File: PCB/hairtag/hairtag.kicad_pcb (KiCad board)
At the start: 2 copper layers, 24 x 24 mm, 19 parts, among them J1 Flash, J2 BAT, U1 ESP32-C3FH4, X1 XL2EL89CPI-111YLC-40M

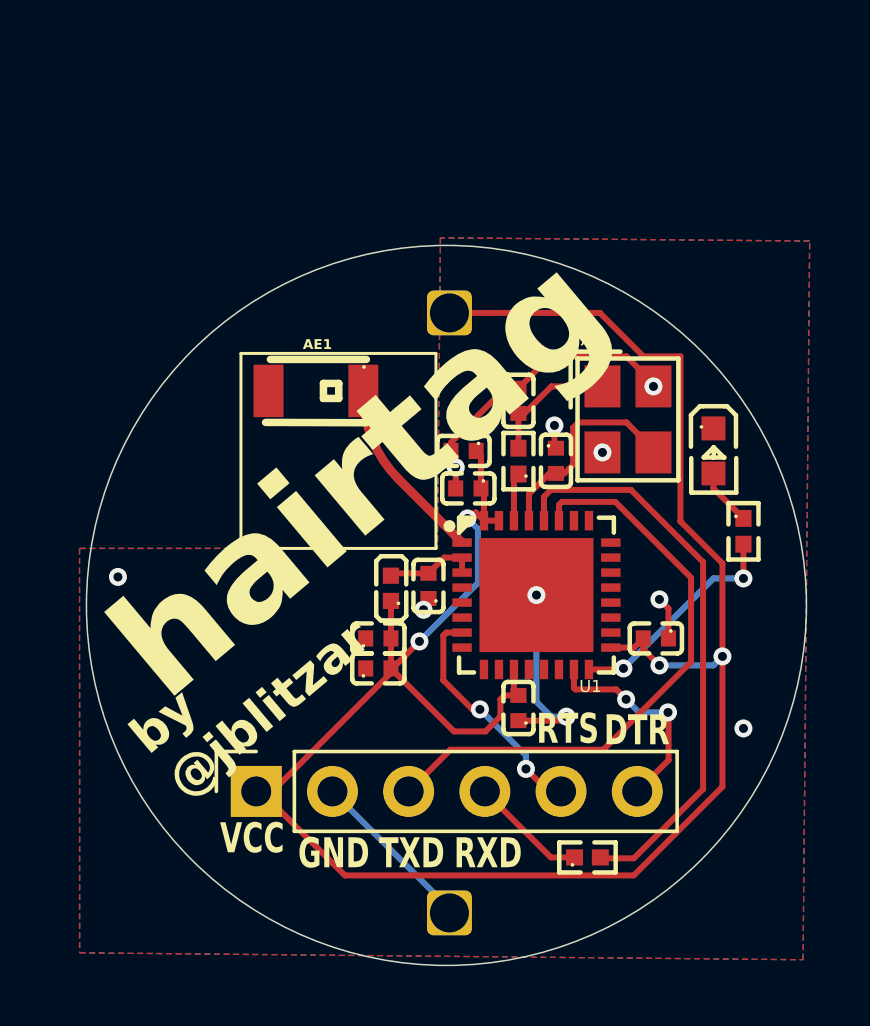
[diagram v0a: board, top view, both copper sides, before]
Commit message: tweaks
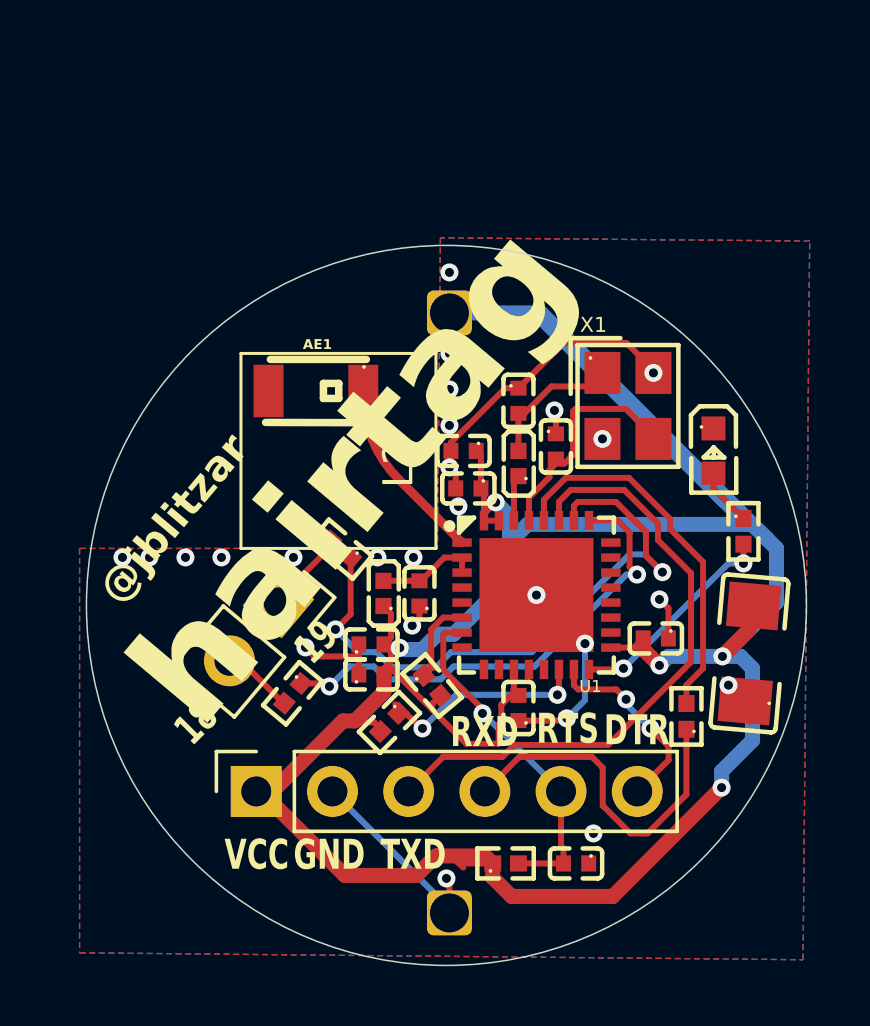
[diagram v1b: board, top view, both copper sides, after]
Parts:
- added C11: 100uF, lcsc:C1206, F.Cu at (65.2, 57.0)
- added C8: 1uF, lcsc:C0402, F.Cu at (59.4, 64.0)
- added L2: 15nH, lcsc:L0402, F.Cu at (57.5, 50.7)
- added R4: 10k, lcsc:R0402, F.Cu at (57.1, 64.0)
- added R5: 10k, lcsc:R0402, F.Cu at (53.2, 59.3)
- added R6: 10k, lcsc:R0402, F.Cu at (54.6, 58.1)
- added R7: 22, lcsc:R0402, F.Cu at (50.0, 58.3)
- added USB1: USB, Connector_PinSocket_2.54mm:PinSocket_1x02_P2.54mm_Vertical, F.Cu at (49.5, 55.3)
- L1: value ~ -> 2nF
- R2: value 24Ω -> 22
- moved R2 6.61 mm to (51.6, 53.5), turned to 140 degrees
- moved R1 5.74 mm to (63.1, 59.1), turned to 90 degrees
- moved C10 0.48 mm to (58.8, 50.1)
- moved X1 0.45 mm to (61.1, 48.8)
- moved C1 0.39 mm to (54.2, 55.0)
- moved C2 0.30 mm to (52.6, 56.7)
- moved C3 0.30 mm to (52.6, 57.7)
- moved L1 0.30 mm to (53.0, 55.0)
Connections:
- R2 pad 1: /XTAL_P -> /GPIO19
- R2 pad 2: Net-(C9-Pad2) -> Net-(USB1-Pin_1)
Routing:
- net /VCC: track 70.0 -> 101.3 mm, vias 4 -> 5
- net /GPIO19: track 0.00 -> 20.8 mm, vias 0 -> 2
- net /GPIO18: track 0.00 -> 16.2 mm, vias 0 -> 2
- net /RXD: track 3.90 -> 11.7 mm
- net /GPIO8: track 0.00 -> 7.05 mm, vias 0 -> 2
- net Net-(U1-U0TXD): track 19.1 -> 12.6 mm
- net /CHIP_EN: track 7.46 -> 11.5 mm, vias 2 -> 1
- net GND: track 24.6 -> 27.6 mm, vias 10 -> 26
- net /GPIO2: track 0.00 -> 2.83 mm
- net Net-(USB1-Pin_1): track 0.00 -> 2.47 mm
- net Net-(USB1-Pin_2): track 0.00 -> 2.00 mm
- net /TXD: track 20.0 -> 20.8 mm
- net /DTR: track 7.16 -> 6.55 mm
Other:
- board text added: "18"
- board text added: "19"
- board text added: "@jblitzar"
- board text removed: "by @jblitzar"
